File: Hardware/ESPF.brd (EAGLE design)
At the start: 30 x 22 mm, 25 parts, among them IC1 CP2102N-A01-GQFN24, J1 USB-C-16P-16P, J2 ESPFLASH-1X6-2.54-PINS-RA, Q1 MMDT3904

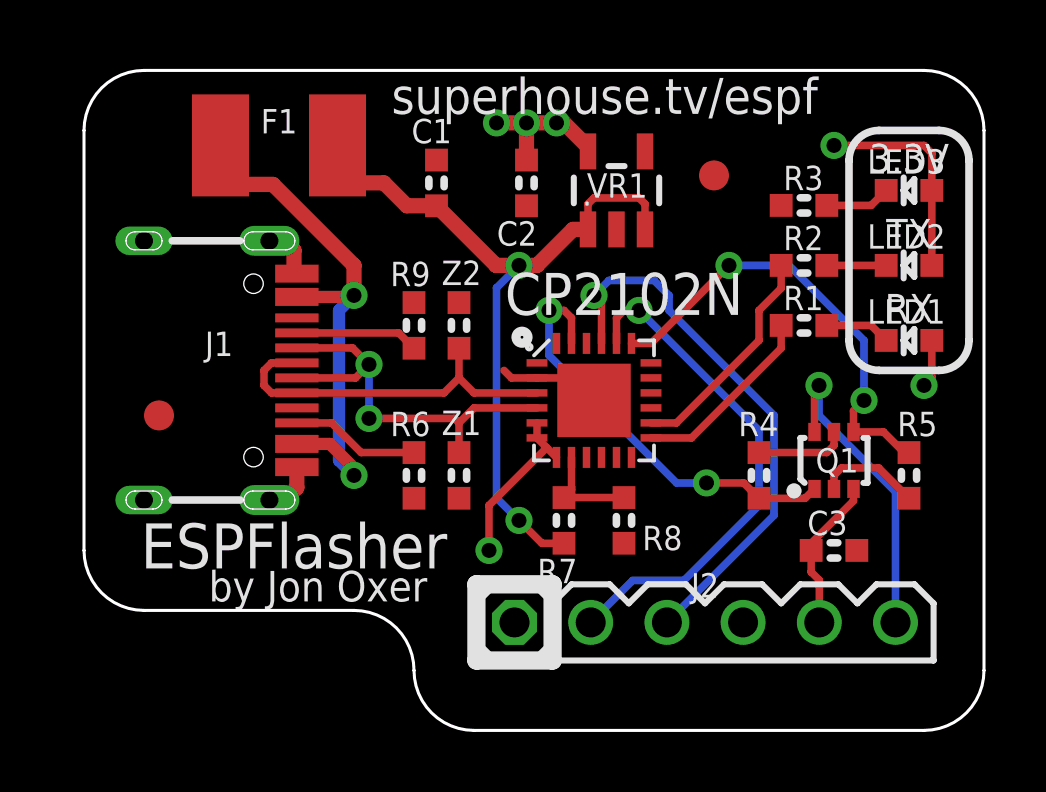
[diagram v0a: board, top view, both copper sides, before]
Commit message: Wurth_Connectors_WR-USB
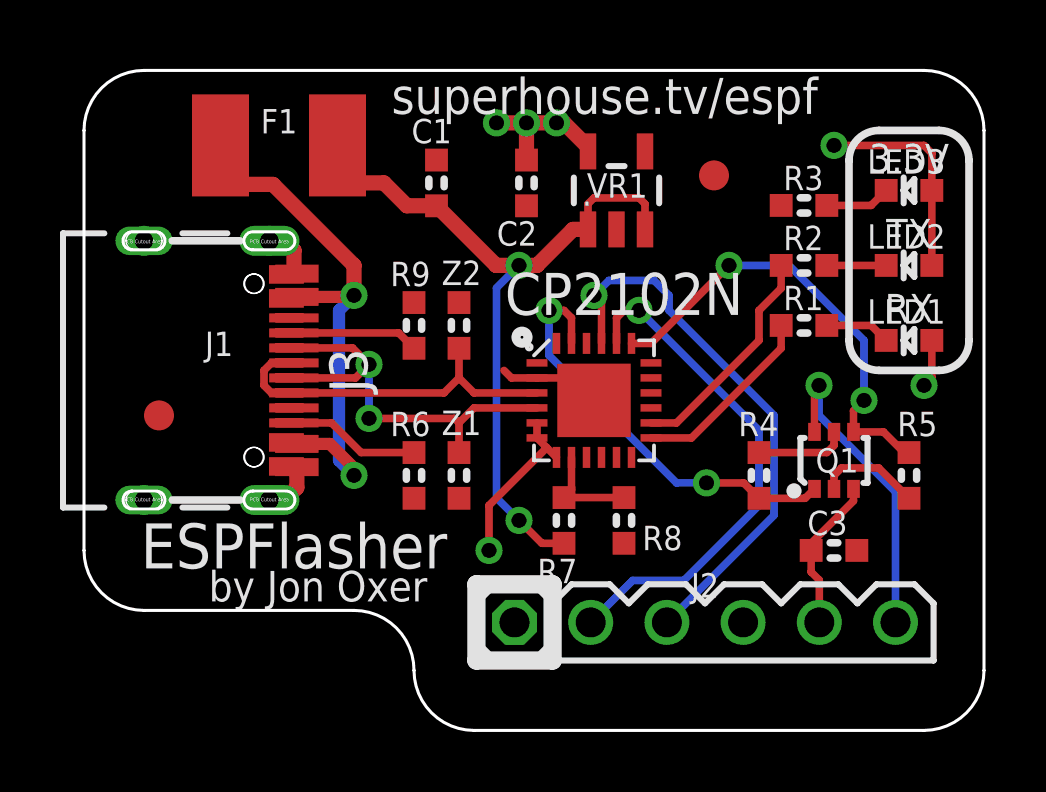
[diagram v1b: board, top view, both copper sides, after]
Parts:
- added J3: 629722000214, Wurth_Connectors_WR-USB:629722000214
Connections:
- removed net VIN: F1.1, J1.A4B9, J1.A9B4
- new net +5V: J3.A4, J3.A9, J3.B4, J3.B9
- net 5V: now also F1.1, J1.A4B9, J1.A9B4
- net D+: now also J3.A7, J3.B7
- net D-: now also J3.A6, J3.B6
- net GND: now also J3.A1, J3.A12, J3.B1, J3.B12
- net N$10: now also J3.A5
- net N$9: now also J3.B5
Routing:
- net VIN: track 18.5 -> 0.00 mm, vias 2 -> 0
- net 5V: track 25.9 -> 44.5 mm, vias 2 -> 4
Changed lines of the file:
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@@
 </layers>
 <board>
-<fusionsync huburn="a.cGVyc29uYWw6dWUyZDliZmNi" projecturn="a.cGVyc29uYWw6dWUyZDliZmNiIzIwMTkwNjE5MTk5NjgzNjgx" f3durn="urn:adsk.wipprod:dm.lineage:swBH170zRHaojB2h5Vblyg" pcbguid="" lastpulledtime="" lastsyncedchangeguid="8f27d1c3-c2be-d358-18db-d89d43a70d9e" latestrevisionid="aa437058-996b-450f-af31-aa14738bf436" lastsyncedrevisionid="aa437058-996b-450f-af31-aa14738bf436" lastboardhashguid="c4cc12bd-3535-9094-fdde-aad7011a1909" lastpushedtime="2021-05-06T07:46:15Z" linktopcb3d="true"/>
+<fusionsync huburn="a.cGVyc29uYWw6dWUyZDliZmNi" projecturn="a.cGVyc29uYWw6dWUyZDliZmNiIzIwMTkwNjE5MTk5NjgzNjgx" f3durn="urn:adsk.wipprod:dm.lineage:swBH170zRHaojB2h5Vblyg" pcbguid="" lastpulledtime="" lastsyncedchangeguid="8f27d1c3-c2be-d358-18db-d89d43a70d9e" latestrevisionid="aa437058-996b-450f-af31-aa14738bf436" lastsyncedrevisionid="aa437058-996b-450f-af31-aa14738bf436" lastboardhashguid="c4cc12bd-3535-9094-fdde-aad7011a1909" lastpushedtime="2021-05-06T07:46:15Z" linktopcb3d="false"/>
 <plain>
 <text x="10.25" y="20.55" size="1.2" layer="21" font="vector" ratio="18">superhouse.tv/espf</text>
@@
 <attribute name="VALUE" x="23.284" y="4.6348" size="0.8128" layer="27" font="vector"/>
 </element>
+<element name="J3" library="Wurth_Connectors_WR-USB" library_urn="urn:adsk.eagle:library:16513831" package="629722000214" package3d_urn="urn:adsk.eagle:package:32827710/4" value="629722000214" x="2" y="12" smashed="yes" rot="R270">
+<attribute name="APPLICATION" value="USB 2.0" x="2" y="12" size="1.778" layer="27" rot="R270" display="off"/>
+<attribute name="DATASHEET-URL" value="https://www.we-online.com/redexpert/spec/629722000214?ae" x="2" y="12" size="1.778" layer="27" rot="R270" display="off"/>
+<attribute name="GERDER" value="Receptacle" x="2" y="12" size="1.778" layer="27" rot="R270" display="off"/>
+<attribute name="INTERFACE-TYPE" value="Type C" x="2" y="12" size="1.778" layer="27" rot="R270" display="off"/>
+<attribute name="IR" value="5A" x="2" y="12" size="1.778" layer="27" rot="R270" display="off"/>
+<attribute name="MOUNT" value="SMT" x="2" y="12" size="1.778" layer="27" rot="R270" display="off"/>
+<attribute name="NAME" x="8.18" y="12" size="1.27" layer="25" rot="R270" align="bottom-center"/>
+<attribute name="PACKAGING" value="Tape and Reel" x="2" y="12" size="1.778" layer="27" rot="R270" display="off"/>
+<attribute name="PART-NUMBER" value="629722000214" x="2" y="12" size="1.778" layer="27" rot="R270" display="off"/>
+<attribute name="PINS" value=" 16 " x="2" y="12" size="1.778" layer="27" rot="R270" display="off"/>
+<attribute name="TYPE" value="Horizontal" x="2" y="12" size="1.778" layer="27" rot="R270" display="off"/>
+<attribute name="VALUE" x="-2.82" y="12" size="1.27" layer="27" rot="R270" align="bottom-center"/>
+<attribute name="WORKING-VOLTAGE" value="20V(AC)" x="2" y="12" size="1.778" layer="27" rot="R270" display="off"/>
+</element>
 </elements>
 <signals>
@@
 <wire x1="11.75" y1="17.488" x2="13.738" y2="15.5" width="0.508" layer="1"/>
 <wire x1="13.738" y1="15.5" x2="14.5" y2="15.5" width="0.508" layer="1"/>
+<contactref element="F1" pad="1"/>
+<contactref element="J1" pad="A4B9"/>
+<contactref element="J1" pad="A9B4"/>
+<wire x1="7.095" y1="9.55" x2="8.19565625" y2="9.55" width="0.4064" layer="1"/>
+<wire x1="9" y1="8.74565625" x2="9" y2="8.5" width="0.4064" layer="1"/>
+<wire x1="8.19565625" y1="9.55" x2="9" y2="8.74565625" width="0.4064" layer="1"/>
+<via x="9" y="8.5" extent="1-16" drill="0.5"/>
+<wire x1="9" y1="8.5" x2="8.5" y2="9" width="0.4064" layer="16"/>
+<wire x1="8.5" y1="14" x2="9" y2="14.5" width="0.4064" layer="16"/>
+<via x="9" y="14.5" extent="1-16" drill="0.5"/>
+<wire x1="9" y1="14.5" x2="8.95" y2="14.45" width="0.4064" layer="1"/>
+<wire x1="8.95" y1="14.45" x2="7.095" y2="14.45" width="0.4064" layer="1"/>
+<wire x1="8.5" y1="9" x2="8.5" y2="14" width="0.4064" layer="16"/>
+<wire x1="9" y1="14.5" x2="9" y2="15.5" width="0.508" layer="1"/>
+<wire x1="4.8" y1="18.2" x2="4.55" y2="18.45" width="0.4064" layer="1"/>
+<wire x1="9" y1="15.5" x2="6.3" y2="18.2" width="0.508" layer="1"/>
+<wire x1="6.3" y1="18.2" x2="4.8" y2="18.2" width="0.508" layer="1"/>
+<wire x1="4.55" y1="18.45" x2="4.55" y2="19.5" width="0.4064" layer="1"/>
+<wire x1="4.55" y1="19.5" x2="8.45" y2="19.5" width="0" layer="19" extent="1-1"/>
 </signal>
 <signal name="GND">
@@
 <wire x1="7.095" y1="8.095" x2="6.68" y2="7.68" width="0.508" layer="1"/>
 <contactref element="C3" pad="2"/>
+<contactref element="J3" pad="A1"/>
+<contactref element="J3" pad="B12"/>
+<contactref element="J3" pad="A12"/>
+<contactref element="J3" pad="B1"/>
 <wire x1="16.75" y1="11.75" x2="17" y2="11" width="0" layer="19" extent="1-1"/>
+<wire x1="6.745" y1="8.65" x2="7.095" y2="8.775" width="0" layer="19" extent="1-1"/>
+<wire x1="7.095" y1="15.225" x2="11" y2="14.262" width="0" layer="19" extent="1-1"/>
+<wire x1="6.745" y1="15.35" x2="7.095" y2="15.225" width="0" layer="19" extent="1-1"/>
+<wire x1="2" y1="16.32" x2="6.18" y2="16.32" width="0" layer="19" extent="1-1"/>
+<wire x1="2" y1="7.68" x2="6.18" y2="7.68" width="0" layer="19" extent="1-1"/>
 </signal>
 <signal name="D-">
@@
 <wire x1="15.1" y1="10.75" x2="13" y2="10.75" width="0.254" layer="1"/>
 <wire x1="13" y1="10.75" x2="12.5" y2="10.25" width="0.254" layer="1"/>
+<contactref element="J3" pad="B6"/>
+<contactref element="J3" pad="A6"/>
+<wire x1="6.745" y1="11.25" x2="7.095" y2="11.75" width="0" layer="19" extent="1-1"/>
+<wire x1="6.745" y1="12.25" x2="7.095" y2="12.75" width="0" layer="19" extent="1-1"/>
 </signal>
 <signal name="D+">
@@
 <wire x1="7.095" y1="11.25" x2="12" y2="11.25" width="0.254" layer="1"/>
 <wire x1="12" y1="11.25" x2="12.5" y2="11.75" width="0.254" layer="1"/>
+<contactref element="J3" pad="A7"/>
+<contactref element="J3" pad="B7"/>
+<wire x1="7.095" y1="12.25" x2="6.745" y2="12.75" width="0" layer="19" extent="1-1"/>
+<wire x1="6.745" y1="11.75" x2="7.095" y2="12.25" width="0" layer="19" extent="1-1"/>
 </signal>
 <signal name="3.3V">
@@
 <wire x1="18.25" y1="12.9" x2="18.9" y2="12.9" width="0.254" layer="1"/>
 </signal>
-<signal name="VIN">
-<contactref element="F1" pad="1"/>
-<contactref element="J1" pad="A4B9"/>
-<contactref element="J1" pad="A9B4"/>
-<wire x1="7.095" y1="9.55" x2="8.19565625" y2="9.55" width="0.4064" layer="1"/>
-<wire x1="9" y1="8.74565625" x2="9" y2="8.5" width="0.4064" layer="1"/>
-<wire x1="8.19565625" y1="9.55" x2="9" y2="8.74565625" width="0.4064" layer="1"/>
-<via x="9" y="8.5" extent="1-16" drill="0.5"/>
-<wire x1="9" y1="8.5" x2="8.5" y2="9" width="0.4064" layer="16"/>
-<wire x1="8.5" y1="14" x2="9" y2="14.5" width="0.4064" layer="16"/>
-<via x="9" y="14.5" extent="1-16" drill="0.5"/>
-<wire x1="9" y1="14.5" x2="8.95" y2="14.45" width="0.4064" layer="1"/>
-<wire x1="8.95" y1="14.45" x2="7.095" y2="14.45" width="0.4064" layer="1"/>
-<wire x1="8.5" y1="9" x2="8.5" y2="14" width="0.4064" layer="16"/>
-<wire x1="9" y1="14.5" x2="9" y2="15.5" width="0.508" layer="1"/>
-<wire x1="4.8" y1="18.2" x2="4.55" y2="18.45" width="0.4064" layer="1"/>
-<wire x1="9" y1="15.5" x2="6.3" y2="18.2" width="0.508" layer="1"/>
-<wire x1="6.3" y1="18.2" x2="4.8" y2="18.2" width="0.508" layer="1"/>
-<wire x1="4.55" y1="18.45" x2="4.55" y2="19.5" width="0.4064" layer="1"/>
-</signal>
 <signal name="N$6">
 <contactref element="R7" pad="1"/>
@@
 <wire x1="9.238" y1="9.262" x2="11" y2="9.262" width="0.254" layer="1"/>
 <wire x1="8.25" y1="10.25" x2="9.238" y2="9.262" width="0.254" layer="1"/>
+<contactref element="J3" pad="B5"/>
+<wire x1="6.745" y1="10.25" x2="7.095" y2="10.25" width="0" layer="19" extent="1-1"/>
 </signal>
 <signal name="N$10">
@@
 <wire x1="7.095" y1="13.25" x2="10.488" y2="13.25" width="0.254" layer="1"/>
 <wire x1="10.488" y1="13.25" x2="11" y2="12.738" width="0.254" layer="1"/>
+<contactref element="J3" pad="A5"/>
+<wire x1="6.745" y1="13.25" x2="7.095" y2="13.25" width="0" layer="19" extent="1-1"/>
+</signal>
+<signal name="+5V">
+<contactref element="J3" pad="A4"/>
+<contactref element="J3" pad="A9"/>
+<contactref element="J3" pad="B4"/>
+<contactref element="J3" pad="B9"/>
+<wire x1="6.745" y1="14.25" x2="6.745" y2="14.55" width="0" layer="19" extent="1-1"/>
+<wire x1="6.745" y1="9.75" x2="6.745" y2="14.25" width="0" layer="19" extent="1-1"/>
+<wire x1="6.745" y1="9.45" x2="6.745" y2="9.75" width="0" layer="19" extent="1-1"/>
 </signal>
 </signals>
